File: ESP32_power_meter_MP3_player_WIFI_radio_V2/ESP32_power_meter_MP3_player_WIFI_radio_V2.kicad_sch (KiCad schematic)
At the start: 78 parts, among them IC1 XRA1203IG24TR-F, J1 STX-3120-5B, J14 Conn_02x10_Odd_Even, J15 I2C, J16 I2C, J2 MEM2051-00-195-00-A, J3 USB_A, J4 Conn_01x06, SW1 GPIO_RESET, SW2 MCU_RESET, U1 LM4040DBZ-3, U2 MCP3208, U3 Adafruit_MAX98357, U4 ESP32-S3-WROOM-1, U5 D1213A-02SM

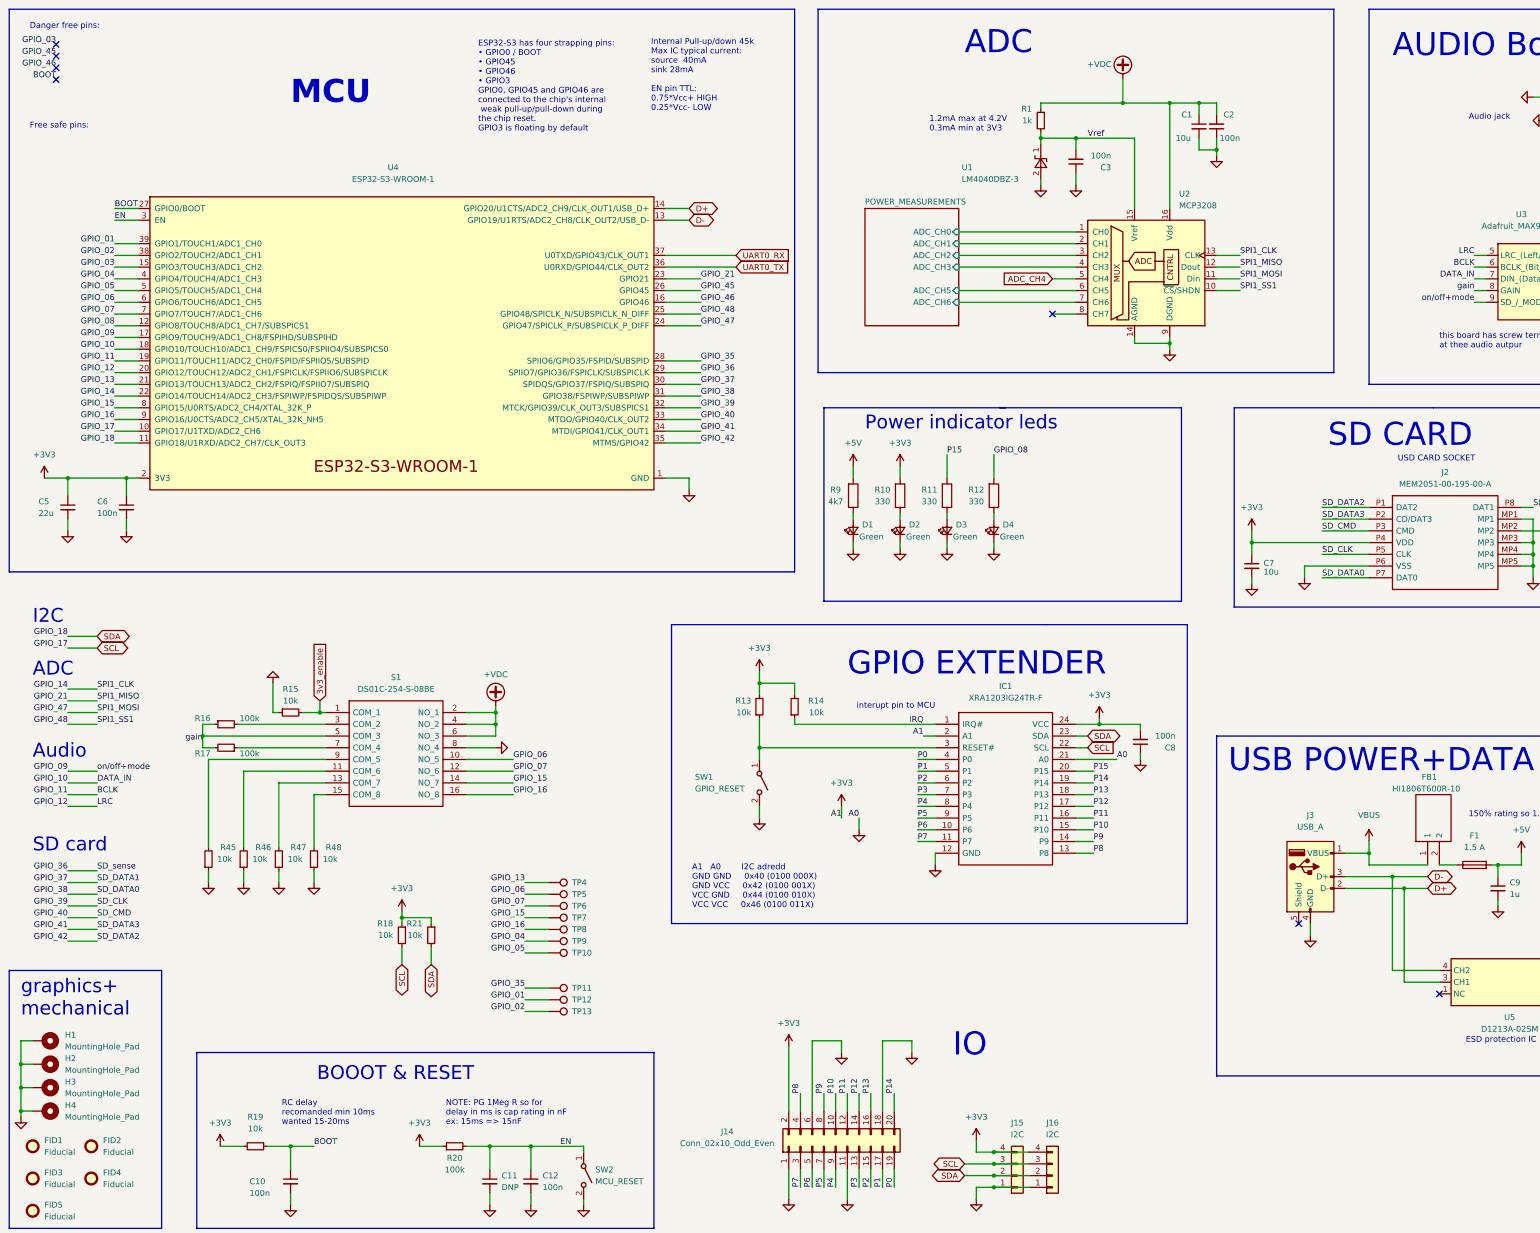
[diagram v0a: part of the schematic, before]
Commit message: f
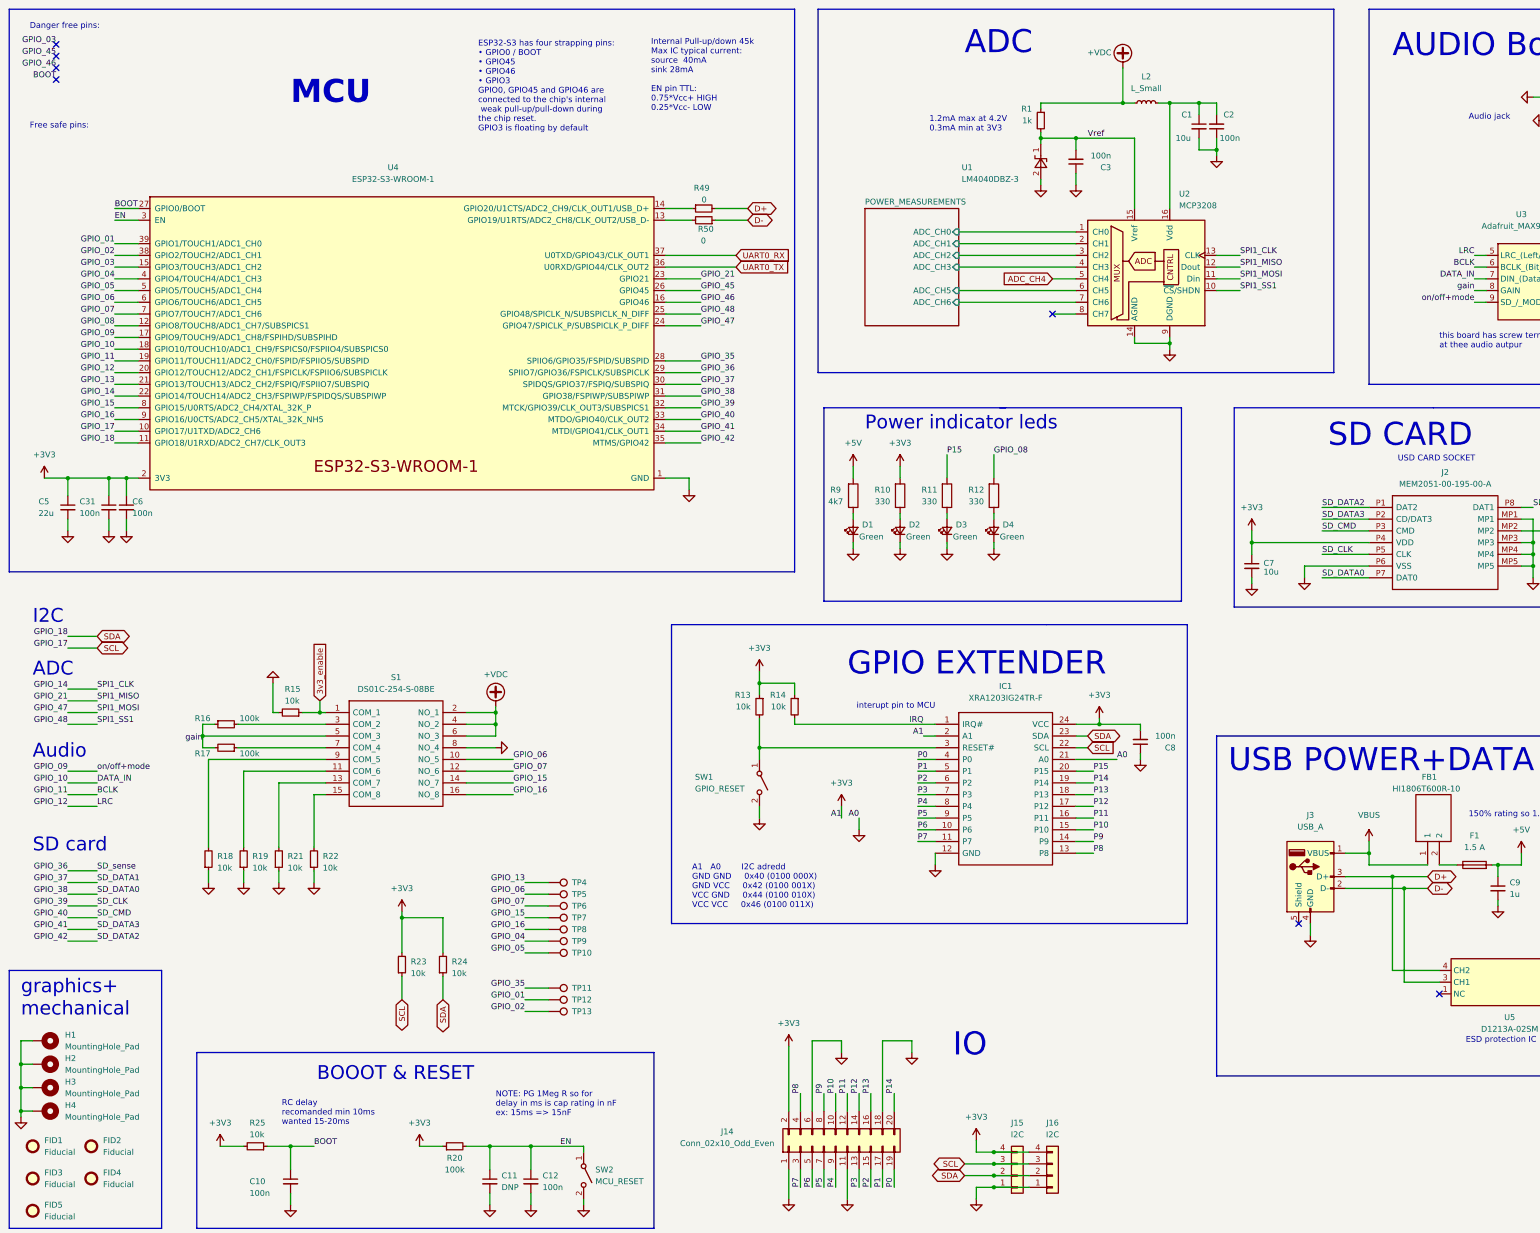
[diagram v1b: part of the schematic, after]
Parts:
- removed R45, R46, R47, R48: 10k, Resistor_SMD:R_0603_1608Metric_Pad0.98x0.95mm_HandSolder, symbol Device:R_Small
- added C31: 100n, Capacitor_SMD:C_0603_1608Metric_Pad1.08x0.95mm_HandSolder, symbol Device:C_Small
- added L2: L_Small, Inductor_SMD:L_1206_3216Metric, symbol Device:L_Small
- added R22, R23, R24, R25: 10k, Resistor_SMD:R_0603_1608Metric, symbol Device:R_Small
- added R49, R50: 0, Resistor_SMD:R_0603_1608Metric_Pad0.98x0.95mm_HandSolder, symbol Device:R_Small
- R13, R14, R15, R18, R19, R2, R21, R3, R4, R5, R6, R7, R8: footprint Resistor_SMD:R_0603_1608Metric_Pad0.98x0.95mm_HandSolder -> Resistor_SMD:R_0603_1608Metric; LCSC (none) -> C25804
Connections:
- net +3V3: now also R13.1, R14.1, C31.1, R23.2, R24.2, R25.2; no longer R13.2, R14.2, R18.1, R19.2, R21.1
- net +VDC: now also L2.1; no longer C1.1, C2.2, U2.16 (Vdd)
- net 3v3_enable: now also R15.1; no longer R15.2
- net BOOT: now also R25.1; no longer R19.1
- net D+: now also J3.3 (D+), U5.4 (CH2), R49.2; no longer J3.2 (D-), U4.14 (GPIO20/U1CTS/ADC2_CH9/CLK_OUT1/USB_D+), U5.3 (CH1)
- net D-: now also J3.2 (D-), U5.3 (CH1), R50.1; no longer J3.3 (D+), U4.13 (GPIO19/U1RTS/ADC2_CH8/CLK_OUT2/USB_D-), U5.4 (CH2)
- net GND: now also R15.2, R18.1, R19.1, R21.1, C31.2, R22.1; no longer R15.1
- net IRQ: now also R14.2; no longer R14.1
- net SCL: now also R23.1; no longer R18.2
- net SDA: now also R24.1; no longer R21.2
- net at IC1.3 (RESET#), SW1.1 (A): now also R13.2; no longer R13.1
- net at S1.13 (COM_7): now also R21.2
- net at S1.11 (COM_6): now also R19.2
- net at S1.9 (COM_5): now also R18.2
- net at S1.15 (COM_8): now also R22.2
- new net: C1.1, C2.2, L2.2, U2.16 (Vdd)
- new net: R49.1, U4.14 (GPIO20/U1CTS/ADC2_CH9/CLK_OUT1/USB_D+)
- new net: R50.2, U4.13 (GPIO19/U1RTS/ADC2_CH8/CLK_OUT2/USB_D-)
